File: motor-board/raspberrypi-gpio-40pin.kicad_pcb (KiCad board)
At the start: 2 copper layers, 81.8 x 38.3 mm, 24 parts, among them J1 Conn_01x15

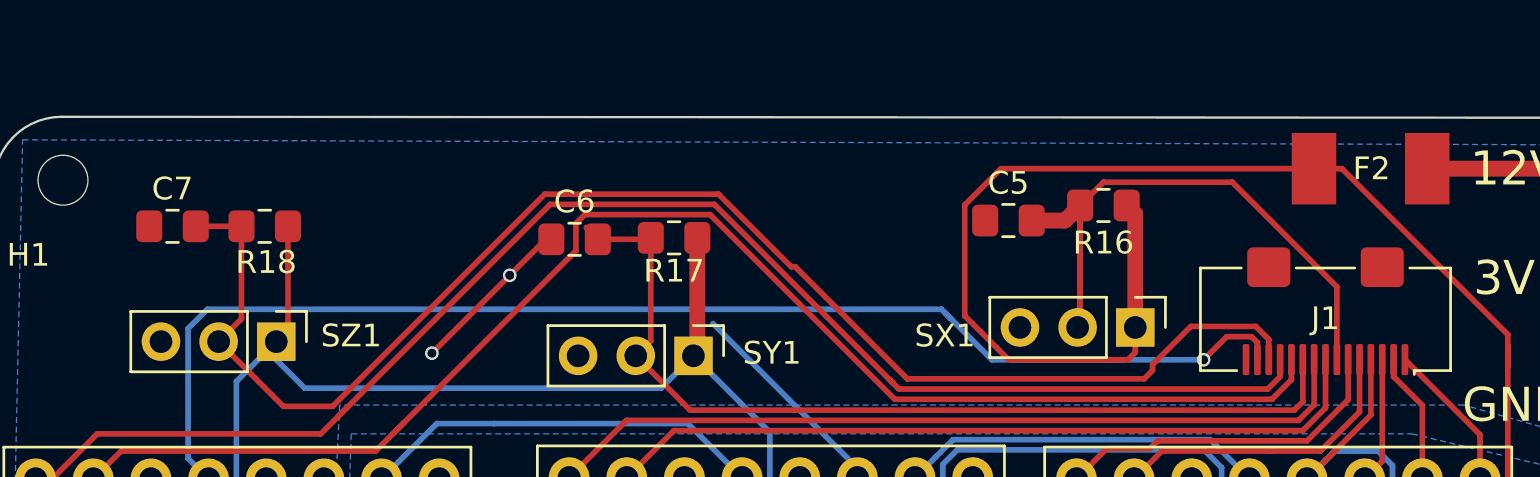
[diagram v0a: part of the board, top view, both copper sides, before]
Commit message: updated bom
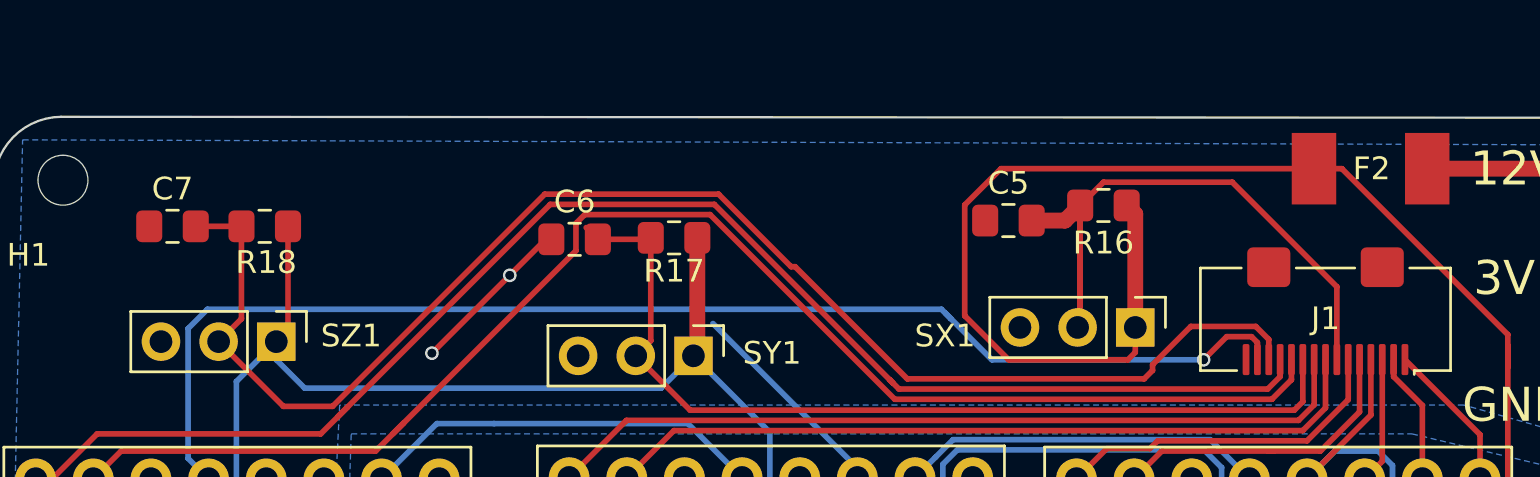
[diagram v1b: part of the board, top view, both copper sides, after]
